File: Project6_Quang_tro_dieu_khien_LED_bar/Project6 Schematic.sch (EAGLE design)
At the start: 16 parts, among them U1 ARDUINOR3-BPLACE

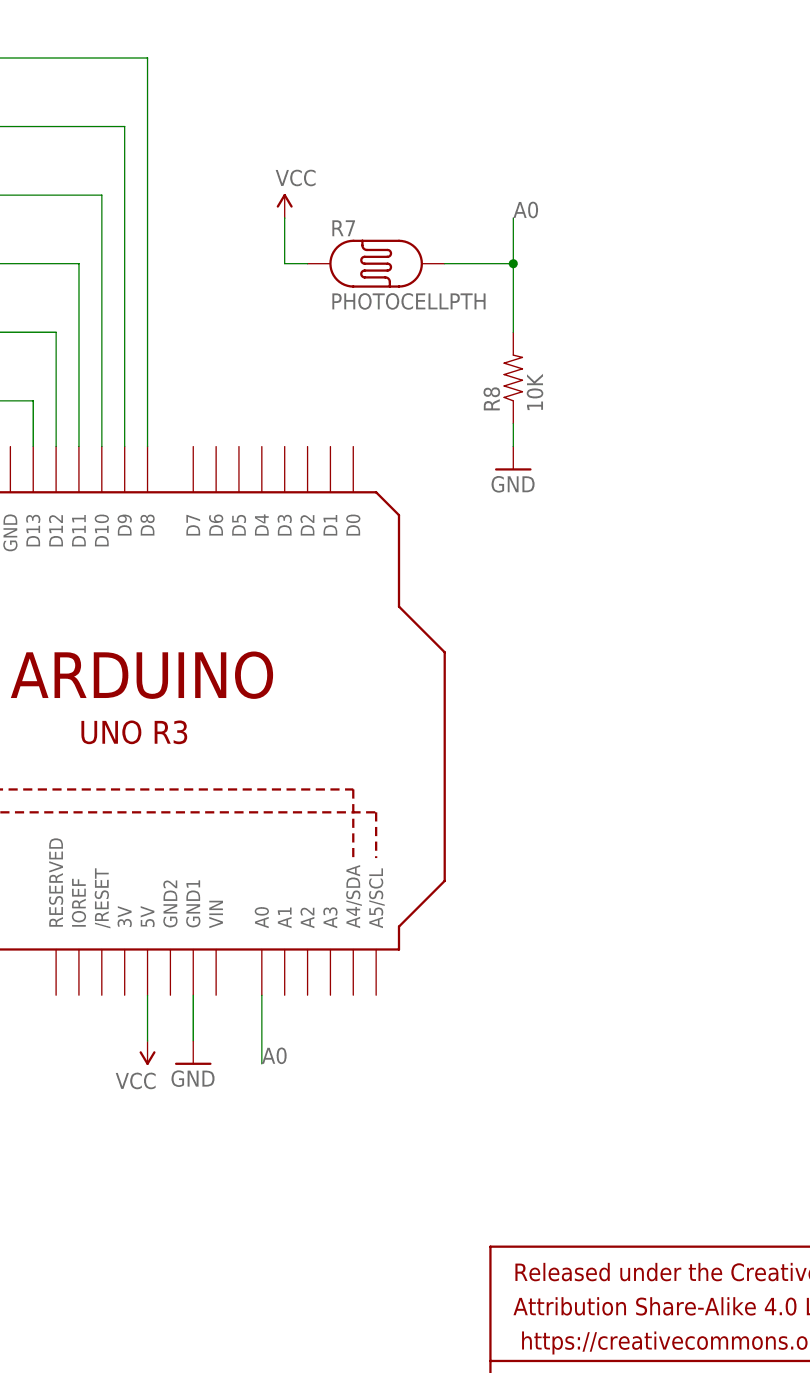
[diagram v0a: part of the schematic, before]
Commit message: Thay doi schematic cua projects.
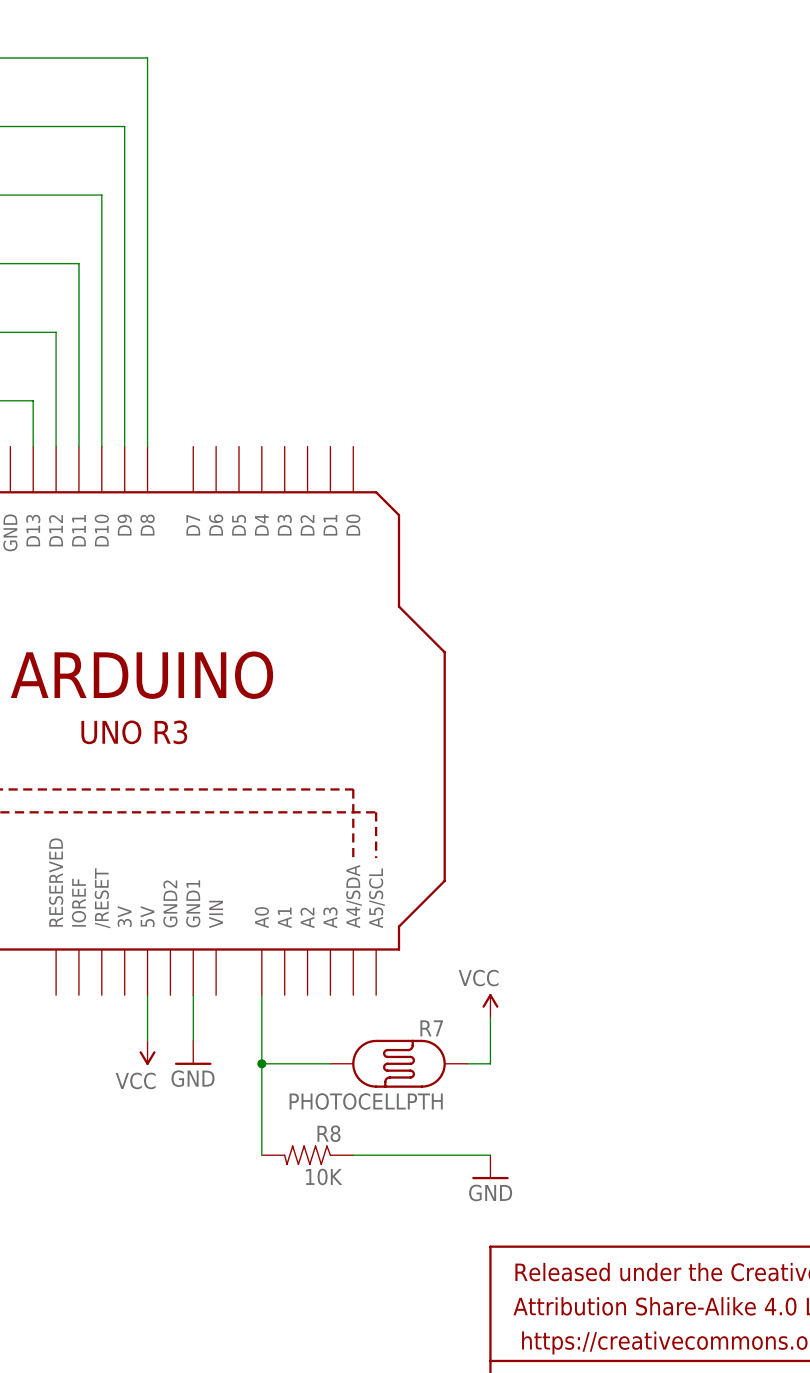
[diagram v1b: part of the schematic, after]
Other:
- moved on the sheet: R7, R8
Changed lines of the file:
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@@
 <?xml version="1.0" encoding="utf-8"?>
 <!DOCTYPE eagle SYSTEM "eagle.dtd">
-<eagle version="7.2.0">
+<eagle version="7.3.0">
 <drawing>
 <settings>
@@
 <instance part="SUPPLY1" gate="G$1" x="76.2" y="43.18" rot="R180"/>
 <instance part="GND1" gate="1" x="81.28" y="40.64"/>
-<instance part="R8" gate="G$1" x="116.84" y="116.84" rot="R90"/>
+<instance part="R8" gate="G$1" x="93.98" y="30.48" rot="MR0"/>
 <instance part="R1" gate="G$1" x="50.8" y="114.3"/>
 <instance part="LED1" gate="G$1" x="38.1" y="114.3" rot="R270"/>
 <instance part="GND2" gate="1" x="27.94" y="109.22"/>
-<instance part="GND3" gate="1" x="116.84" y="106.68"/>
-<instance part="SUPPLY2" gate="G$1" x="91.44" y="134.62"/>
+<instance part="GND3" gate="1" x="114.3" y="27.94" rot="MR0"/>
+<instance part="SUPPLY2" gate="G$1" x="114.3" y="45.72" rot="MR0"/>
 <instance part="FRAME1" gate="G$1" x="-33.02" y="-15.24"/>
 <instance part="FRAME1" gate="V" x="114.3" y="-15.24"/>
@@
 <instance part="R2" gate="G$1" x="50.8" y="121.92"/>
 <instance part="R3" gate="G$1" x="50.8" y="129.54"/>
-<instance part="R7" gate="G$1" x="101.6" y="129.54"/>
+<instance part="R7" gate="G$1" x="104.14" y="40.64" rot="MR0"/>
 <instance part="LED4" gate="G$1" x="38.1" y="137.16" rot="R270"/>
 <instance part="LED5" gate="G$1" x="38.1" y="144.78" rot="R270"/>
@@
 <segment>
 <pinref part="SUPPLY2" gate="G$1" pin="VCC"/>
-<wire x1="91.44" y1="134.62" x2="91.44" y2="129.54" width="0.1524" layer="91"/>
+<wire x1="114.3" y1="45.72" x2="114.3" y2="40.64" width="0.1524" layer="91"/>
 <pinref part="R7" gate="G$1" pin="P$1"/>
-<wire x1="91.44" y1="129.54" x2="93.98" y2="129.54" width="0.1524" layer="91"/>
+<wire x1="114.3" y1="40.64" x2="111.76" y2="40.64" width="0.1524" layer="91"/>
 </segment>
 </net>
@@
 <pinref part="R8" gate="G$1" pin="1"/>
 <pinref part="GND3" gate="1" pin="GND"/>
-<wire x1="116.84" y1="111.76" x2="116.84" y2="109.22" width="0.1524" layer="91"/>
+<wire x1="99.06" y1="30.48" x2="114.3" y2="30.48" width="0.1524" layer="91"/>
 </segment>
 </net>
@@
 <segment>
 <pinref part="R7" gate="G$1" pin="P$2"/>
-<wire x1="109.22" y1="129.54" x2="116.84" y2="129.54" width="0.1524" layer="91"/>
+<wire x1="96.52" y1="40.64" x2="88.9" y2="40.64" width="0.1524" layer="91"/>
 <pinref part="R8" gate="G$1" pin="2"/>
-<wire x1="116.84" y1="129.54" x2="116.84" y2="121.92" width="0.1524" layer="91"/>
-<wire x1="116.84" y1="129.54" x2="116.84" y2="134.62" width="0.1524" layer="91"/>
-<junction x="116.84" y="129.54"/>
-<label x="116.84" y="134.62" size="1.778" layer="95"/>
-</segment>
-<segment>
+<wire x1="88.9" y1="40.64" x2="88.9" y2="30.48" width="0.1524" layer="91"/>
 <pinref part="U1" gate="G$1" pin="A0"/>
 <wire x1="88.9" y1="48.26" x2="88.9" y2="40.64" width="0.1524" layer="91"/>
-<label x="88.9" y="40.64" size="1.778" layer="95"/>
-</segment>
-</net>
+<junction x="88.9" y="40.64"/>
+</segment>
+</net>
